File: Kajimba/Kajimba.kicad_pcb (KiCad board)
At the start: 2 copper layers, 69.8 x 46.2 mm, 24 parts, among them J1 Barrel_Jack_Switch, J2 Pump, J3 Sensor, J4 Screen, J5 Button, K1 Relay, Q1 BSS138, Q2 BSS138, SW1 Button, U1 Pico, U2 LM78M05

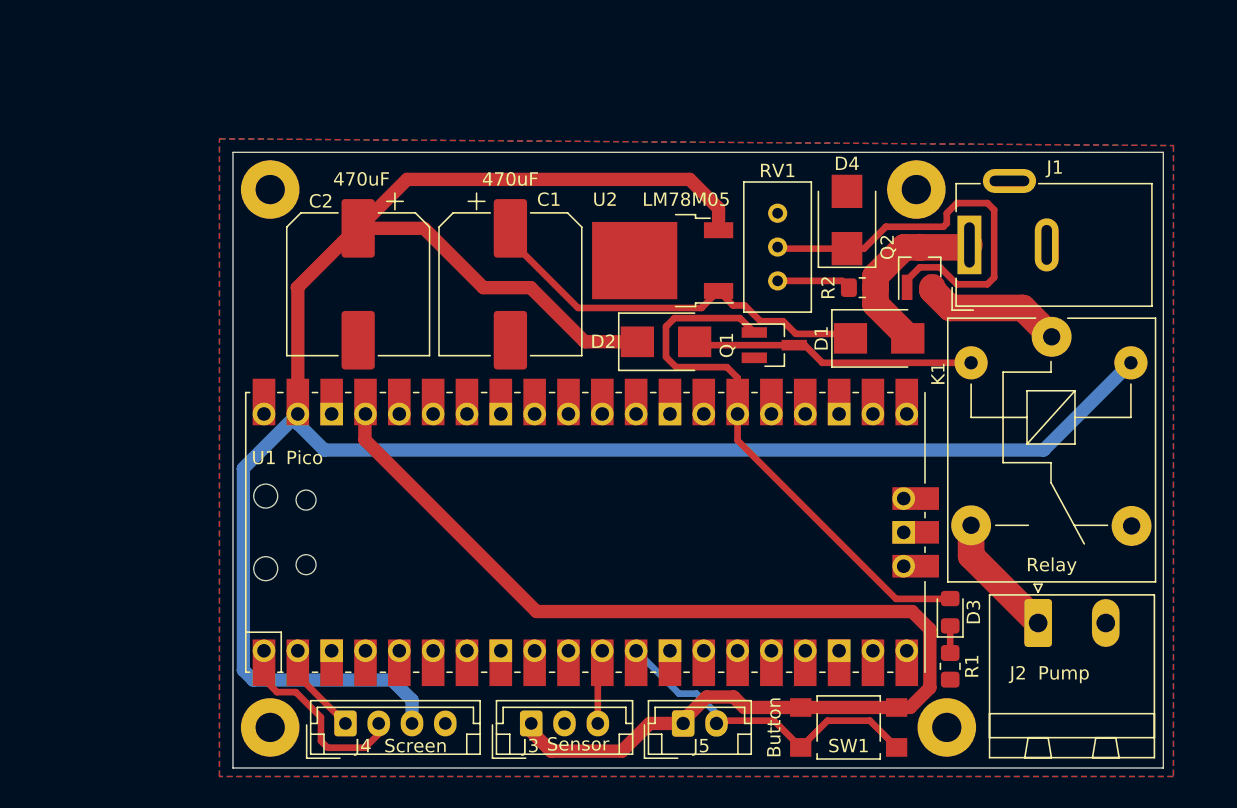
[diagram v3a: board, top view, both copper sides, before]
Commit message: KiCad PCB Pump v04
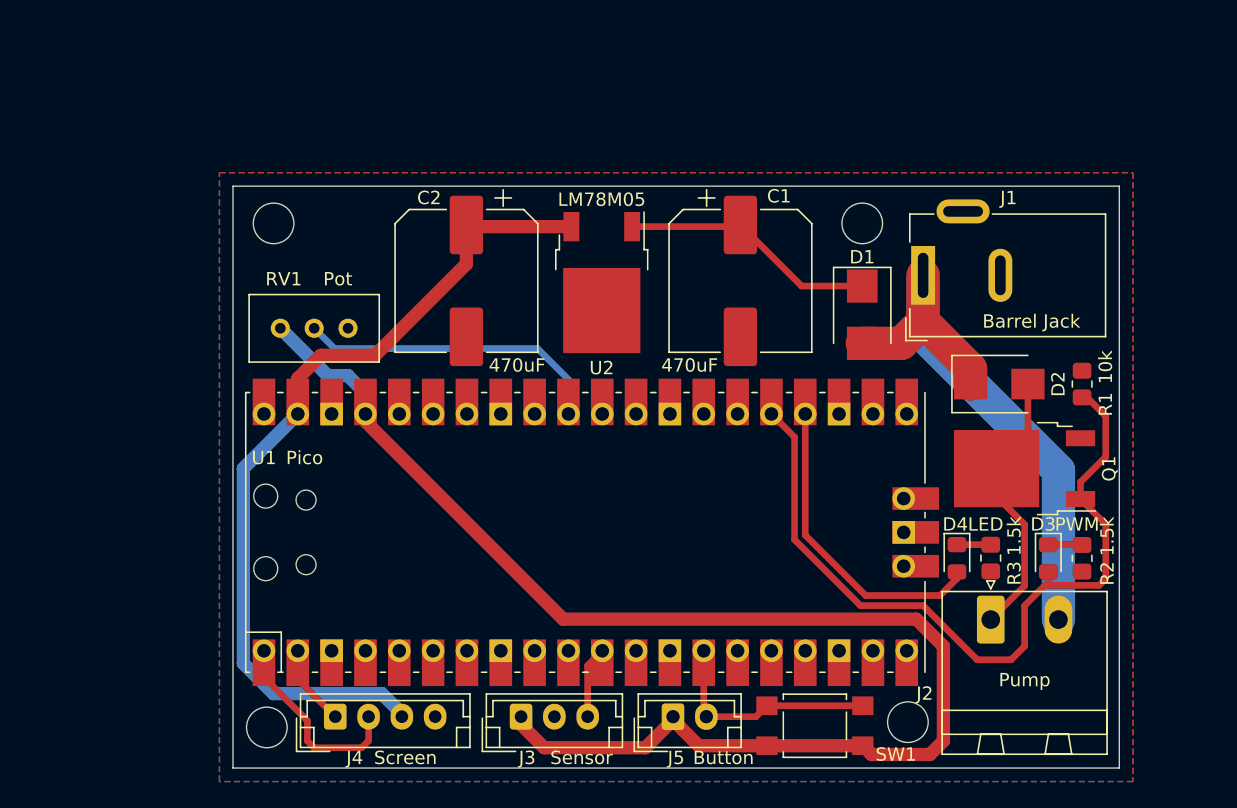
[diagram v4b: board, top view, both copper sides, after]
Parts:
- removed H1, H2, H3, H4: GND_Pad, MountingHole:MountingHole_2.2mm_M2_Pad
- removed K1: Relay, Relay_THT:Relay_SPDT_SANYOU_SRD_Series_Form_C
- removed Q2: BSS138, Package_TO_SOT_SMD:SOT-23_Handsoldering
- removed the R2 at (160.5, 87.4)
- added R1: 10k, Resistor_SMD:R_0805_2012Metric_Pad1.20x1.40mm_HandSolder, F.Cu at (177.0, 94.6)
- added R3: 1.5k, Resistor_SMD:R_0805_2012Metric_Pad1.20x1.40mm_HandSolder, F.Cu at (170.2, 107.7)
- D4: value S2JTR -> RED; footprint Diode_SMD:D_SMB -> LED_SMD:LED_0805_2012Metric_Pad1.15x1.40mm_HandSolder
- J1: value Barrel_Jack_Switch -> Barrel Jack
- Q1: value BSS138 -> QM6006D; footprint Package_TO_SOT_SMD:SOT-23_Handsoldering -> Package_TO_SOT_SMD:TO-252-2
- RV1: value R_Potentiometer -> Pot
- moved RV1 32.5 mm to (121.9, 90.4), turned to 0 degrees
- moved D4 26.7 mm to (167.6, 107.7), turned to -90 degrees
- moved D2 25.2 mm to (170.8, 94.6)
- moved Q1 21.0 mm to (172.7, 101.0), turned to 180 degrees
- moved C1 17.3 mm to (151.4, 86.9)
- moved R2 12.8 mm to (177.0, 107.7)
- moved D3 8.41 mm to (174.5, 107.7), turned to -90 degrees
- moved C2 8.13 mm to (130.8, 86.9)
- moved U2 4.86 mm to (141.0, 87.0), turned to -90 degrees
- moved J1 4.16 mm to (165.1, 86.5)
- moved J2 3.57 mm to (170.2, 112.3)
- moved SW1 2.54 mm to (157.0, 120.3), turned to 0 degrees
- moved D1 2.18 mm to (160.5, 89.4), turned to -90 degrees
- moved J3 0.92 mm to (134.9, 119.6)
- moved J4 0.92 mm to (121.0, 119.6)
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- renumbered R1 to R2
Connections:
- D2 pad 1: +5V -> +12V
- D3 pad 2: Relay -> PWM
- D4 pad 2: GND -> LED
- J2 pad 1: Net-(J2-Pad1) -> Net-(D2-Pad2)
- J2 pad 2: GND -> +12V
- Q1 pad 1: Relay -> PWM
- Q1 pad 2: GND -> Net-(D2-Pad2)
- Q1 pad 3: Net-(D2-Pad2) -> GND
- RV1 pad 1: Net-(R2-Pad1) -> GND
- RV1 pad 2: Net-(D4-Pad1) -> Analog
- RV1 pad 3: GND -> +3.3V
- U1 pad 12: Button -> unconnected-(U1-Pad12)
- U1 pad 14: unconnected-(U1-Pad14) -> Button
- U1 pad 24: unconnected-(U1-Pad24) -> LED
- U1 pad 25: unconnected-(U1-Pad25) -> PWM
- U1 pad 31: unconnected-(U1-Pad31) -> Analog
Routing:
- net +5V: track 174.6 -> 64.3 mm
- net PWM: track 0.00 -> 58.8 mm
- net Relay: track 41.2 -> 0.00 mm
- net +12V: track 13.7 -> 44.9 mm
- net Net-(D4-Pad1): track 31.7 -> 2.54 mm
- net LED: track 0.00 -> 23.4 mm
- net Analog: track 0.00 -> 23.3 mm
- net +3.3V: track 88.6 -> 103.7 mm
- net Net-(C1-Pad1): track 30.5 -> 19.2 mm
- net Pump: track 10.6 -> 0.00 mm
- net Net-(J2-Pad1): track 9.42 -> 0.00 mm
- net Button: track 25.2 -> 17.1 mm
- net Net-(R2-Pad1): track 5.56 -> 0.00 mm
- net SCL: track 6.94 -> 8.50 mm
- net Net-(D3-Pad1): track 2.04 -> 2.59 mm
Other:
- board size 69.8 x 46.2 mm -> 66.5 x 43.7 mm
- board text added: "LED"
- board text added: "PWM"
- board text added: "v04 Kajimba Pump"
- board text removed: "v03 Kajimba Pump"
